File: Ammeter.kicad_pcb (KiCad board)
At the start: 2 copper layers, 20.3 x 10.8 mm, 16 parts, among them J1 Conn_01x08, U1 INA226

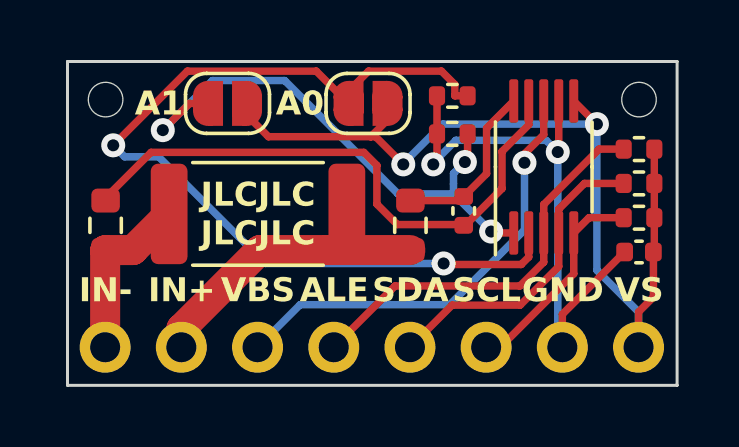
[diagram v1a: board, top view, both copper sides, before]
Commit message: Add files via upload
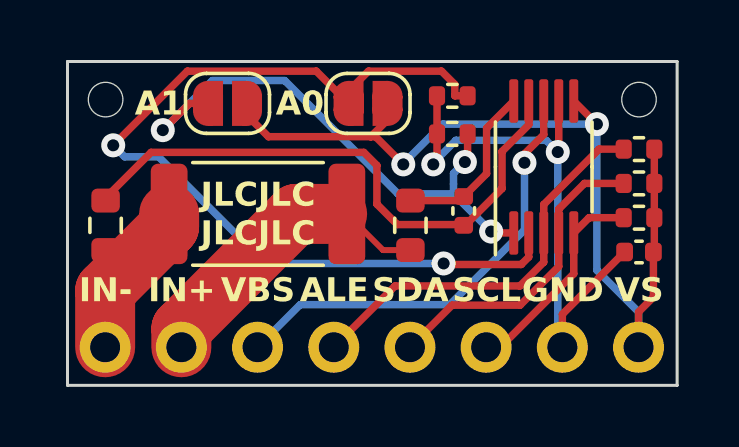
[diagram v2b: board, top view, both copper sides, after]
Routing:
- net VIN-: track 5.86 -> 7.95 mm
- net VIN+: track 10.6 -> 10.0 mm
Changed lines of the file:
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@@
   (segment (start 157.242497 94.234) (end 157.242497 94.208198) (width 0.25) (layer "B.Cu") (net 10))
   (segment (start 163.6974 97.7655) (end 163.6974 92.8924) (width 0.25) (layer "B.Cu") (net 10))
-  (segment (start 154.6841 97.091) (end 155.575 97.091) (width 1) (layer "F.Cu") (net 11))
-  (segment (start 152.464 97.091) (end 154.6841 97.091) (width 1) (layer "F.Cu") (net 11))
-  (segment (start 149.845 100.33) (end 149.845 99.71) (width 1) (layer "F.Cu") (net 11))
-  (segment (start 149.845 99.71) (end 152.464 97.091) (width 1) (layer "F.Cu") (net 11))
-  (segment (start 155.575 97.091) (end 157.48 97.091) (width 1) (layer "F.Cu") (net 11))
-  (segment (start 155.3625 95.885) (end 155.3625 96.8785) (width 1) (layer "F.Cu") (net 11))
-  (segment (start 155.3625 96.8785) (end 155.575 97.091) (width 1) (layer "F.Cu") (net 11))
-  (segment (start 149.4375 95.8855) (end 149.4375 95.885) (width 0.25) (layer "F.Cu") (net 12))
-  (segment (start 149.438 95.885) (end 149.4375 95.8855) (width 1) (layer "F.Cu") (net 12))
-  (segment (start 149.4375 95.8855) (end 148.232 97.091) (width 1) (layer "F.Cu") (net 12))
-  (segment (start 148.232 97.091) (end 147.32 97.091) (width 1) (layer "F.Cu") (net 12))
-  (segment (start 147.305 97.106) (end 147.32 97.091) (width 1) (layer "F.Cu") (net 12))
-  (segment (start 147.305 100.33) (end 147.305 97.106) (width 1) (layer "F.Cu") (net 12))
+  (segment (start 149.845 100.33) (end 149.845 99.71) (width 2) (layer "F.Cu") (net 11))
+  (segment (start 155.3625 95.885) (end 156.5685 97.091) (width 0.2) (layer "F.Cu") (net 11))
+  (segment (start 156.5685 97.091) (end 157.48 97.091) (width 0.2) (layer "F.Cu") (net 11))
+  (segment (start 153.67 95.885) (end 155.0375 95.885) (width 2) (layer "F.Cu") (net 11))
+  (segment (start 149.845 99.71) (end 153.67 95.885) (width 2) (layer "F.Cu") (net 11))
+  (segment (start 147.305 100.33) (end 147.305 98.44) (width 2) (layer "F.Cu") (net 12))
+  (segment (start 147.32 97.091) (end 148.2315 97.091) (width 0.2) (layer "F.Cu") (net 12))
+  (segment (start 149.4375 96.3075) (end 149.4375 95.885) (width 2) (layer "F.Cu") (net 12))
+  (segment (start 148.2315 97.091) (end 149.4375 95.885) (width 0.2) (layer "F.Cu") (net 12))
+  (segment (start 147.305 98.44) (end 149.4375 96.3075) (width 2) (layer "F.Cu") (net 12))
 )
